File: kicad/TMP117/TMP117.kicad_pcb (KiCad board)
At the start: 2 copper layers, 7.8 x 6.4 mm, 7 parts, among them J1 Conn, J2 Conn, J3 Conn, J4 Conn

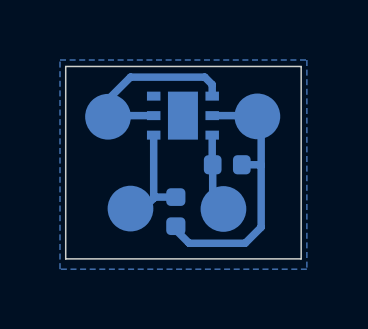
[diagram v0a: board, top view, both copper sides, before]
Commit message: изменено:      kicad/TMP117/TMP117-cache.lib 	изменено:      kicad/TMP117/TMP117.kicad_pcb 	изменено:      kicad/TMP117/TMP117.kicad_pcb-bak 	изменено:      kicad/TMP117/TMP117.sch 	изменено:      kicad/TMP117/TMP117.sch-bak
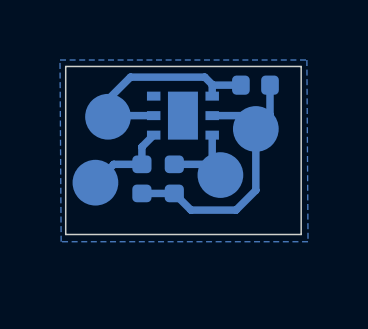
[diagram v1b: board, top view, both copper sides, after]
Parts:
- added C1: C, Capacitor_SMD:C_0402_1005Metric, B.Cu at (49.7, 44.5)
- moved R1 1.83 mm to (47.0, 47.7), turned to 90 degrees
- moved R2 1.57 mm to (45.9, 47.7)
- moved J2 1.45 mm to (44.4, 47.8)
- moved J3 1.13 mm to (48.5, 47.5)
- moved J1 0.42 mm to (49.7, 46.0)
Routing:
- net GND: track 6.38 -> 7.35 mm
- net Net-(D1-Pad1): track 3.78 -> 2.94 mm
- net Net-(D1-Pad6): track 2.62 -> 3.13 mm
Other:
- board size 7.8 x 6.4 mm -> 7.8 x 5.6 mm

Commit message: изменено:      kicad/TMP117/TMP117-cache.lib 	изменено:      kicad/TMP117/TMP117.kicad_pcb 	изменено:      kicad/TMP117/TMP117.kicad_pcb-bak 	изменено:      kicad/TMP117/TMP117.sch 	изменено:      kicad/TMP117/TMP117.sch-bak
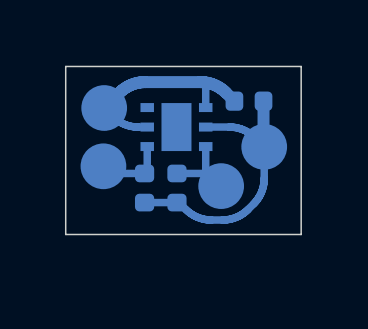
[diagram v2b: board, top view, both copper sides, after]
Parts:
- moved J1 0.66 mm to (50.0, 46.6)
- moved J2 0.61 mm to (44.6, 47.2)
- moved C1 0.58 mm to (49.5, 45.1)
- moved D1 0.44 mm to (47.1, 45.9)
- moved J3 0.37 mm to (48.6, 47.9)
- moved J4 0.32 mm to (44.7, 45.3)
- moved R1 0.32 mm to (47.1, 48.0)
- moved R2 0.32 mm to (46.0, 48.0)
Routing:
- net Net-(D1-Pad1): track 2.94 -> 2.40 mm
- removed copper zone on B.Cu, net GND

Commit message: изменено:      kicad/TMP117/TMP117-cache.lib 	изменено:      kicad/TMP117/TMP117.kicad_pcb 	изменено:      kicad/TMP117/TMP117.kicad_pcb-bak 	изменено:      kicad/TMP117/TMP117.sch 	изменено:      kicad/TMP117/TMP117.sch-bak
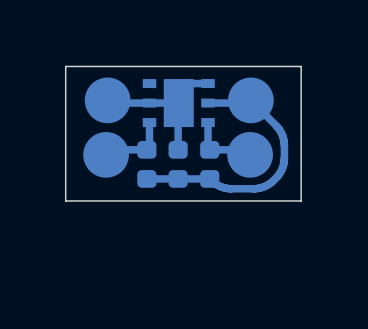
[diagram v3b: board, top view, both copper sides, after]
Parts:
- C1: value C -> 0.1uF
- J1: value Conn -> Vcc
- J2: value Conn -> SCL
- J3: value Conn -> SDA
- J4: value Conn -> GND
- R1, R2: value 5k -> 5.1k
- moved C1 3.17 mm to (47.1, 47.2), turned to 90 degrees
- moved J1 1.61 mm to (49.6, 45.0)
- moved J3 1.42 mm to (49.5, 46.9)
- moved R1 1.35 mm to (48.2, 47.2)
- moved D1 0.80 mm to (47.2, 45.1)
- moved R2 0.79 mm to (46.1, 47.2)
- moved J2 0.39 mm to (44.7, 46.9)
- moved J4 0.28 mm to (44.8, 45.0)
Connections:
- net +3V3 renamed Net-(C1-Pad1)
- D1 pad 7: (no net) -> GND
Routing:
- net GND: track 7.40 -> 5.54 mm
- net Net-(D1-Pad6): track 3.18 -> 2.35 mm
- net Net-(C1-Pad1): track 9.70 -> 9.06 mm
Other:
- board size 7.8 x 5.6 mm -> 7.8 x 4.5 mm
